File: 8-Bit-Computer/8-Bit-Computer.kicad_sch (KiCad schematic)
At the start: 260 parts, among them IC1 AT28C64B-15SU-T, IC2 AT28C64B-15SU-T, IC3 AT28C64B-15SU-T, SW1 SW_Push, SW2 SW_DIP_x04, SW3 SW_DIP_x08, SW4 SW_Push, SW5 SW_Push, SW6 SW_Push_DPDT, SW7 SW_Push_DPDT, SW8 SW_Push_DPDT, U1 NA555D, U10 74LS283, U11 74HC245, U12 74HC86, U13 74HC86, U14 74HC245, U15 HM62256BLP, U16 74HC245, U17 74157, U18 74157, U19 74157, U2 AMS1117-5.0, U20 74HC00, U21 74157, U22 D1X8K-14BL, U23 74LS377, U24 74LS377, U25 74LS377, U26 74HC245, U27 74LS161, U28 74HC245, U29 74LS377, U3 74HC00, U30 D1X8K-14BL, U31 74LS377, U32 D1X8K-14BL, U34 74LS107, U35 NA555D, U36 74LS139, U37 74LS161, U38 74LS138, U39 74LS08, U4 NA555D, U40 74LS04, U41 74LS04, U42 74LS377, U43 74LS00, U44 D1X8K-14BL, U5 NA555D, U6 74HC00, U7 74HC245, U8 74LS02, U9 74LS283

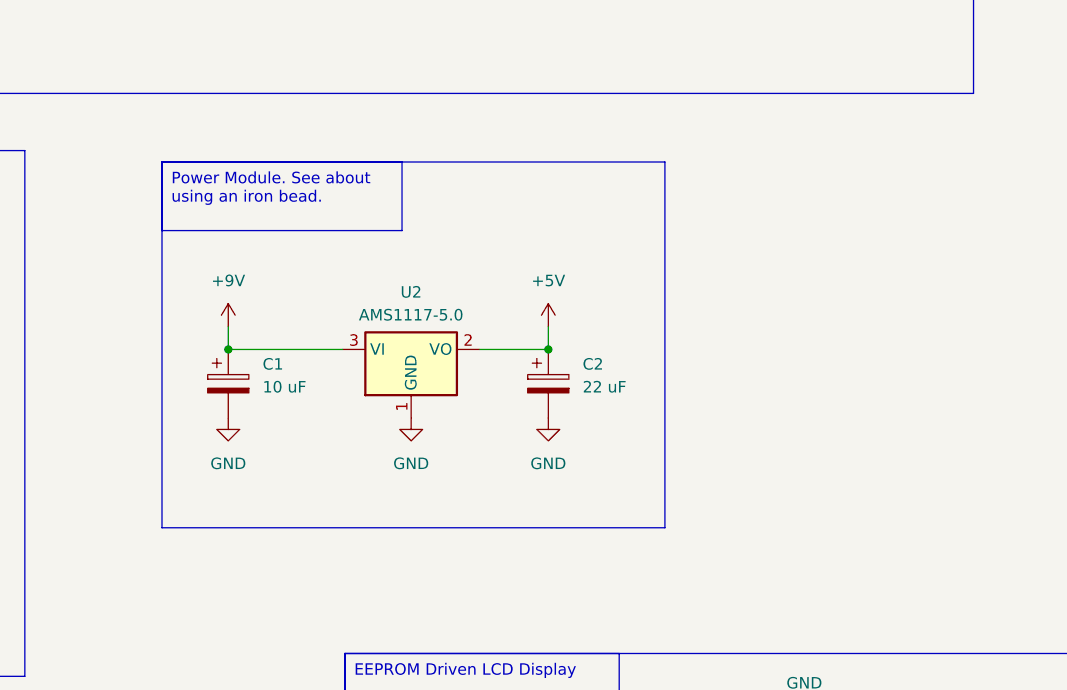
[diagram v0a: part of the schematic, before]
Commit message: Created Gerber Files
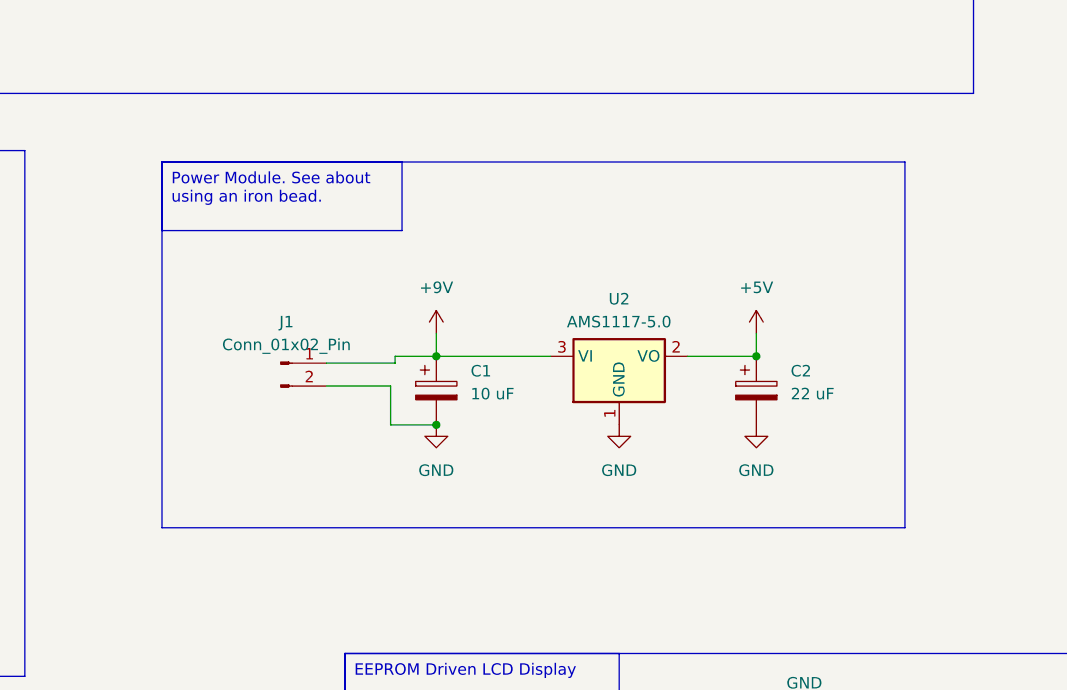
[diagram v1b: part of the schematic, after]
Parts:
- added J1: Conn_01x02_Pin, Connector_PinSocket_2.54mm:PinSocket_1x02_P2.54mm_Vertical, symbol Connector:Conn_01x02_Pin
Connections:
- net +9V: now also J1.1 (Pin_1)
- net GND: now also J1.2 (Pin_2)
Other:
- moved on the sheet: C1, C2, U2
